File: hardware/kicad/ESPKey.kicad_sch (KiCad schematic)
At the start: 32 parts, among them P1 Power, P2 Wiegand, Q1 2N7002, Q2 2N7002, Q3 2N7002, U1 RT6212A/B, U2 ESP-12

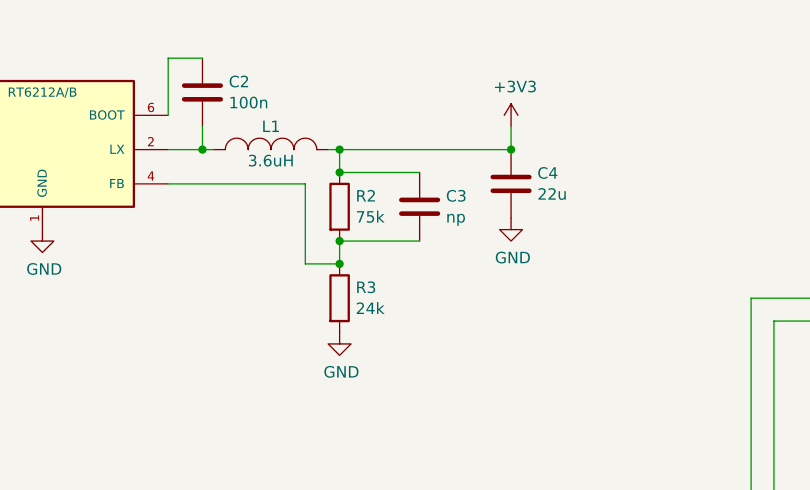
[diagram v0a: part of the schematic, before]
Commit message: Remove unused component C3
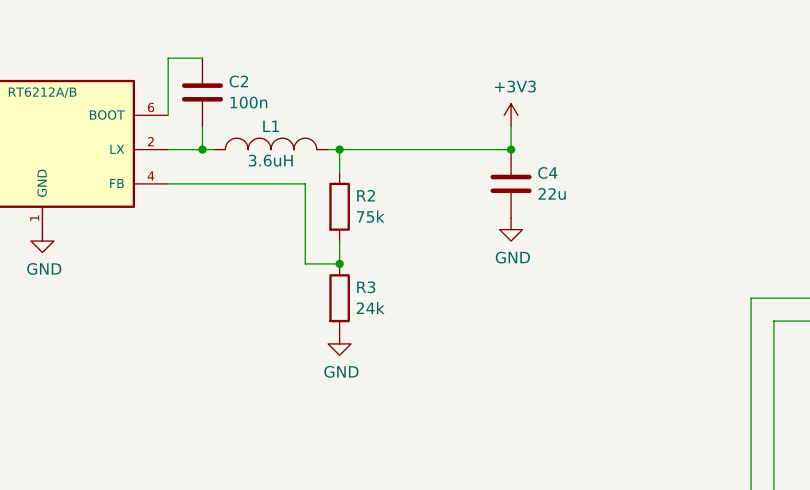
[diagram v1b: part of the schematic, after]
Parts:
- removed C3: np, Capacitors_SMD:C_0402, symbol ESPKey-rescue:C
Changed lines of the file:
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@@
 	)
 	(junction
-		(at 114.3 46.99)
-		(diameter 0)
-		(color 0 0 0 0)
-	)
-	(junction
 		(at 114.3 36.83)
 		(diameter 0)
@@
 	)
 	(junction
-		(at 114.3 39.37)
-		(diameter 0)
-		(color 0 0 0 0)
-	)
-	(junction
 		(at 151.13 106.68)
 		(diameter 0)
@@
 	(wire
 		(pts
-			(xy 123.19 46.99) (xy 114.3 46.99)
-		)
-		(stroke
-			(width 0)
-			(type default)
-		)
-	)
-	(wire
-		(pts
 			(xy 60.96 36.83) (xy 64.77 36.83)
 		)
@@
 	(wire
 		(pts
-			(xy 123.19 39.37) (xy 114.3 39.37)
-		)
-		(stroke
-			(width 0)
-			(type default)
-		)
-	)
-	(wire
-		(pts
 			(xy 36.83 101.6) (xy 186.69 101.6)
 		)
@@
 					(unit 1)
 				)
-			)
-		)
-	)
-	(symbol
-		(lib_name "C_7")
-		(lib_id "ESPKey-rescue:C")
-		(at 123.19 43.18 180)
-		(unit 1)
-		(exclude_from_sim no)
-		(in_bom yes)
-		(on_board yes)
-		(dnp no)
-		(property "Reference" "C3"
-			(at 126.111 42.0116 0)
-			(effects
-				(font
-					(size 1.27 1.27)
-				)
-				(justify right)
-			)
-		)
-		(property "Value" "np"
-			(at 126.111 44.3484 0)
-			(effects
-				(font
-					(size 1.27 1.27)
-				)
-				(justify right)
-			)
-		)
-		(property "Footprint" "Capacitors_SMD:C_0402"
-			(at 122.2248 39.37 0)
-			(effects
-				(font
-					(size 1.27 1.27)
-				)
-				(hide yes)
-			)
-		)
-		(property "Datasheet" ""
-			(at 123.19 43.18 0)
-			(effects
-				(font
-					(size 1.27 1.27)
-				)
-			)
-		)
-		(property "Description" ""
-			(at 123.19 43.18 0)
-			(effects
-				(font
-					(size 1.27 1.27)
-				)
-			)
-		)
-		(pin "1"
-		)
-		(pin "2"
-		)
-		(instances
-			(project ""
-				(path "/1f33d41d-661d-4049-af44-ba9af8c3ad9e"
-					(reference "C3")
-					(unit 1)
-				)

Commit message: Revert R1, R2, R3 to 0402 and C3
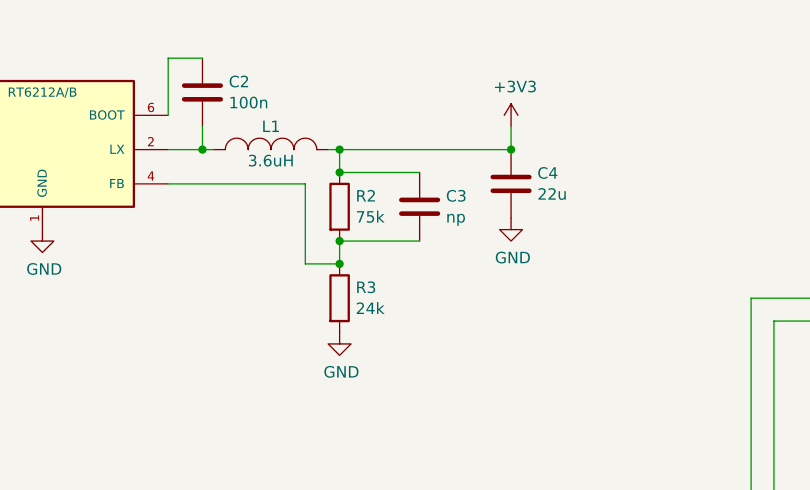
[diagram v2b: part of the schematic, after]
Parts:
- added C3: np, Capacitors_SMD:C_0402, symbol ESPKey-rescue:C
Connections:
- net +3V3: now also C3.2
- net at R2.2, R3.1, U1.4 (FB): now also C3.1
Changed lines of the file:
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@@
 	)
 	(junction
+		(at 114.3 46.99)
+		(diameter 0)
+		(color 0 0 0 0)
+	)
+	(junction
 		(at 114.3 36.83)
 		(diameter 0)
@@
 	)
 	(junction
+		(at 114.3 39.37)
+		(diameter 0)
+		(color 0 0 0 0)
+	)
+	(junction
 		(at 151.13 106.68)
 		(diameter 0)
@@
 	(wire
 		(pts
+			(xy 123.19 46.99) (xy 114.3 46.99)
+		)
+		(stroke
+			(width 0)
+			(type default)
+		)
+	)
+	(wire
+		(pts
 			(xy 60.96 36.83) (xy 64.77 36.83)
 		)
@@
 	(wire
 		(pts
+			(xy 123.19 39.37) (xy 114.3 39.37)
+		)
+		(stroke
+			(width 0)
+			(type default)
+		)
+	)
+	(wire
+		(pts
 			(xy 36.83 101.6) (xy 186.69 101.6)
 		)
@@
 					(unit 1)
 				)
+			)
+		)
+	)
+	(symbol
+		(lib_name "C_7")
+		(lib_id "ESPKey-rescue:C")
+		(at 123.19 43.18 180)
+		(unit 1)
+		(exclude_from_sim no)
+		(in_bom yes)
+		(on_board yes)
+		(dnp no)
+		(property "Reference" "C3"
+			(at 126.111 42.0116 0)
+			(effects
+				(font
+					(size 1.27 1.27)
+				)
+				(justify right)
+			)
+		)
+		(property "Value" "np"
+			(at 126.111 44.3484 0)
+			(effects
+				(font
+					(size 1.27 1.27)
+				)
+				(justify right)
+			)
+		)
+		(property "Footprint" "Capacitors_SMD:C_0402"
+			(at 122.2248 39.37 0)
+			(effects
+				(font
+					(size 1.27 1.27)
+				)
+				(hide yes)
+			)
+		)
+		(property "Datasheet" ""
+			(at 123.19 43.18 0)
+			(effects
+				(font
+					(size 1.27 1.27)
+				)
+			)
+		)
+		(property "Description" ""
+			(at 123.19 43.18 0)
+			(effects
+				(font
+					(size 1.27 1.27)
+				)
+			)
+		)
+		(pin "1"
+		)
+		(pin "2"
+		)
+		(instances
+			(project ""
+				(path "/1f33d41d-661d-4049-af44-ba9af8c3ad9e"
+					(reference "C3")
+					(unit 1)
+				)
